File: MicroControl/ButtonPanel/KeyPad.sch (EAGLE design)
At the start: 15 parts

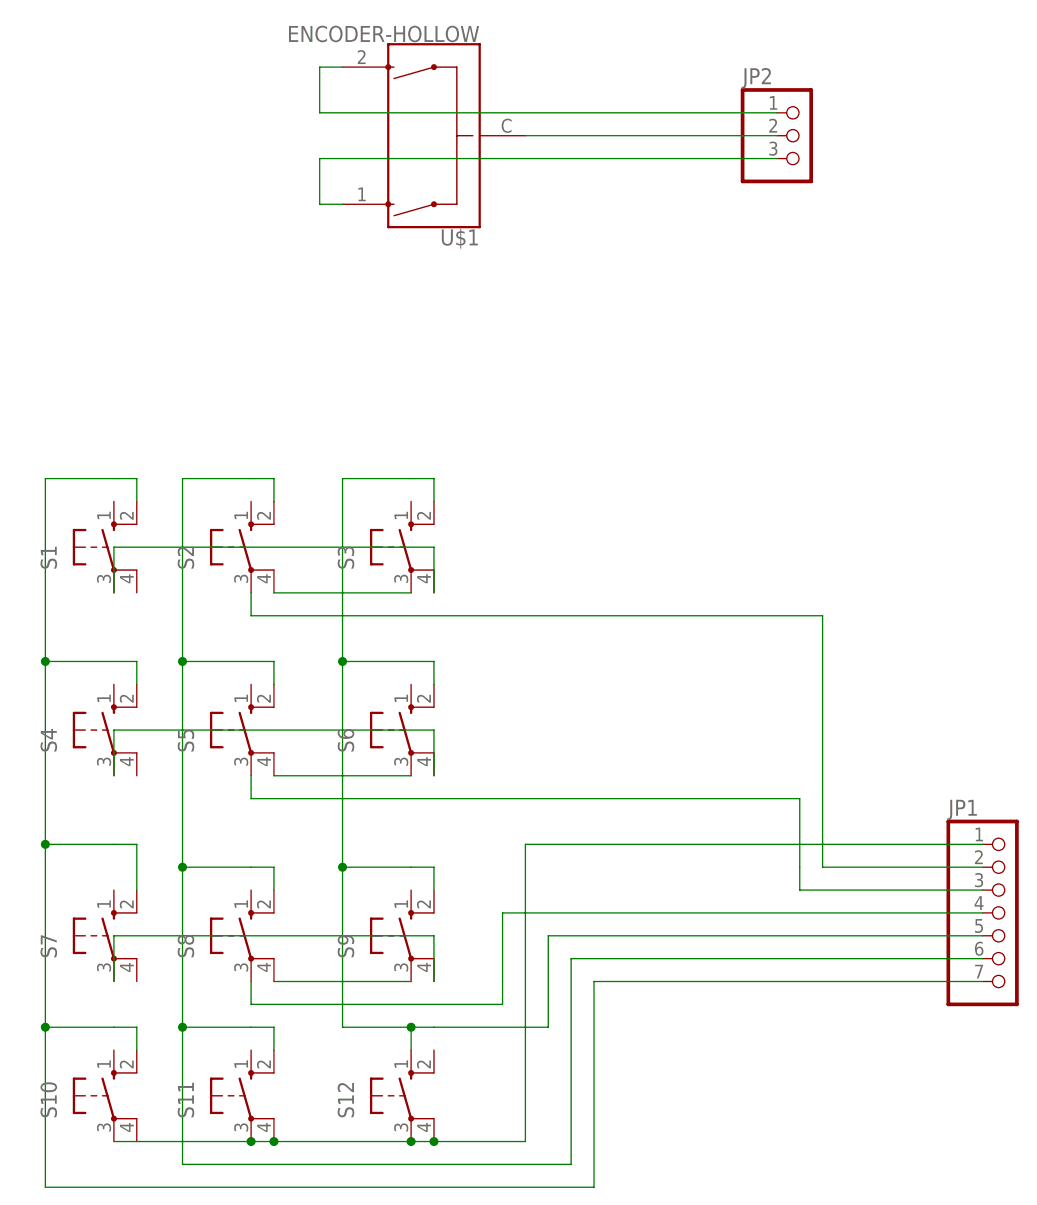
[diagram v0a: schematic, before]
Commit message: more accurate
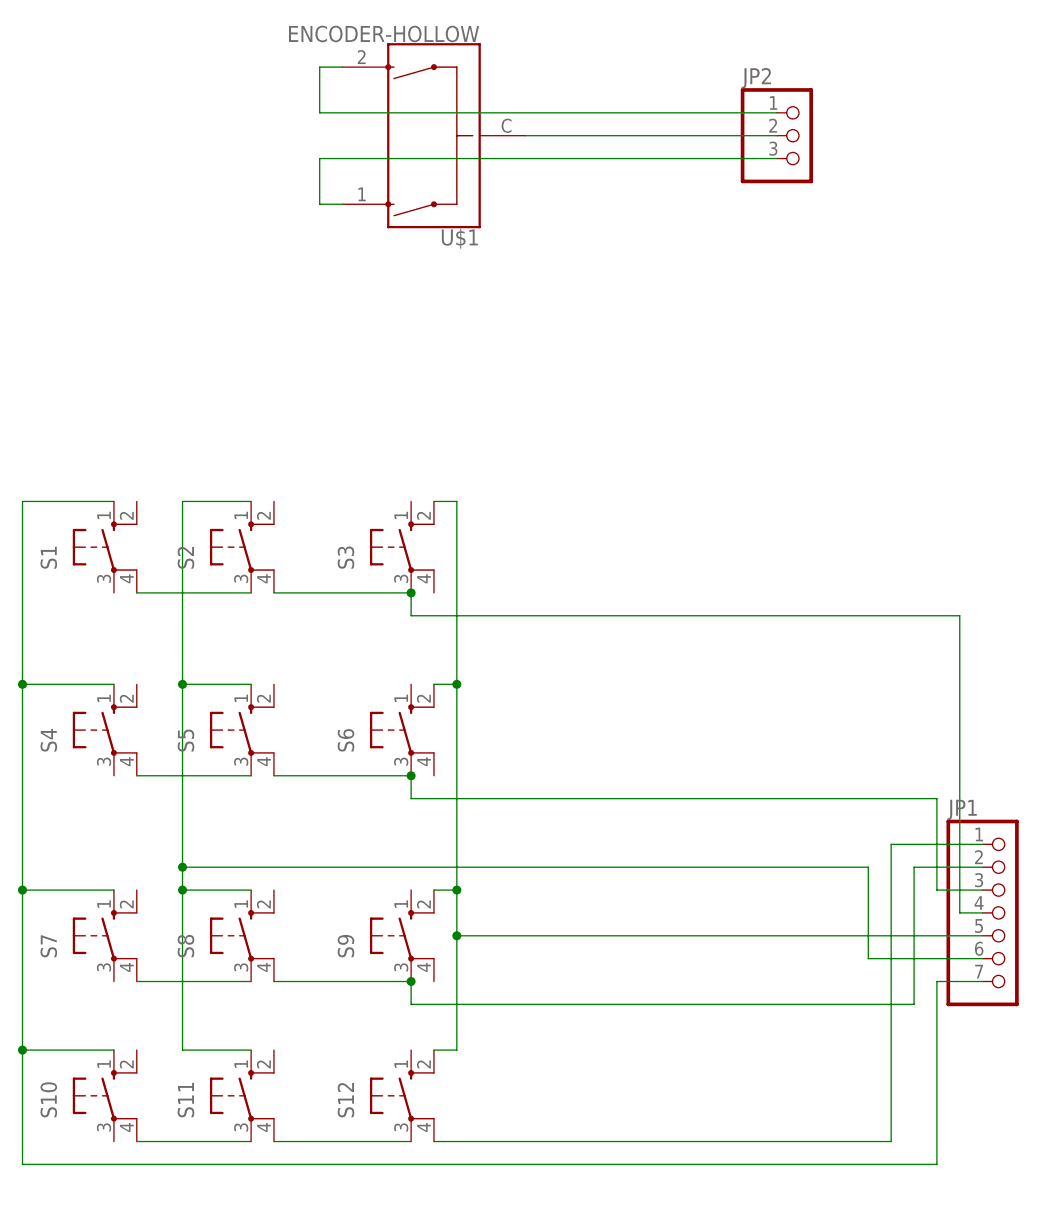
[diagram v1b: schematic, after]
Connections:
- removed net N$16: S1.P, S3.P1
- net N$10: now also S1.P1, S2.P; no longer JP1.6, S11.S1, S2.S1, S5.S1, S8.S1
- net N$11: now also JP1.4, S2.P1, S3.P; no longer S7.P, S9.P1
- net N$12: now also JP1.1, S12.P1; no longer S5.P1, S6.P
- net N$13: now also JP1.7, S1.S, S10.S, S4.S, S7.S; no longer JP1.5, S12.S, S3.S1, S6.S1, S9.S1
- net N$14: now also JP1.6, S11.S, S2.S, S5.S, S8.S; no longer S4.P, S6.P1
- net N$15: now also JP1.5, S12.S1, S3.S1, S6.S1, S9.S1; no longer S2.P1, S3.P
- net N$4: now also S10.P1, S11.P; no longer JP1.2, S2.P
- net N$5: now also S11.P1, S12.P; no longer JP1.3, S5.P
- net N$6: now also JP1.2, S8.P1, S9.P; no longer JP1.4, S8.P
- net N$7: now also S7.P1, S8.P; no longer JP1.1, S10.P, S11.P, S11.P1, S12.P, S12.P1
- net N$8: now also S4.P1, S5.P; no longer JP1.7, S1.S1, S10.S1, S4.S1, S7.S1
- net N$9: now also JP1.3, S5.P1, S6.P; no longer S8.P1, S9.P
